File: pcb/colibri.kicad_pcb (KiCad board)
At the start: 2 copper layers, 160 x 95.2 mm, 97 parts

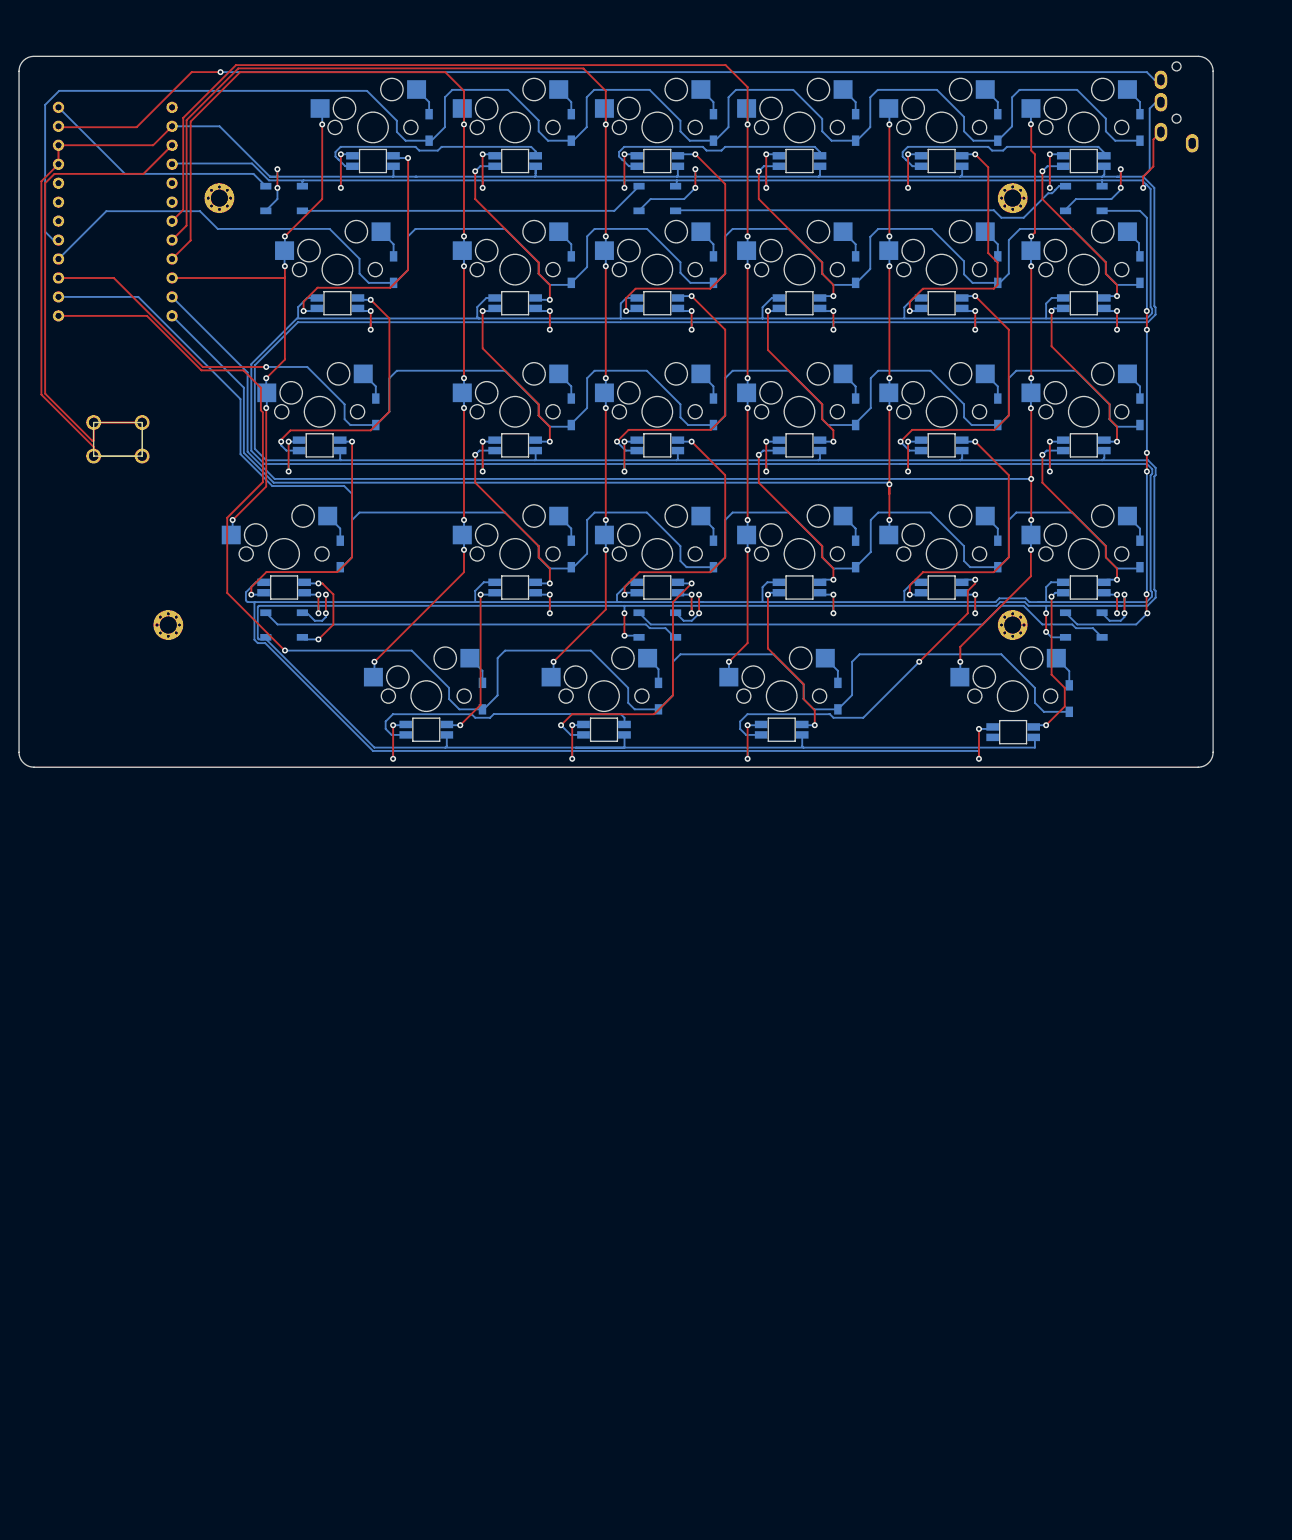
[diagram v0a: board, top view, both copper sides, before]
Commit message: starting to build the right side
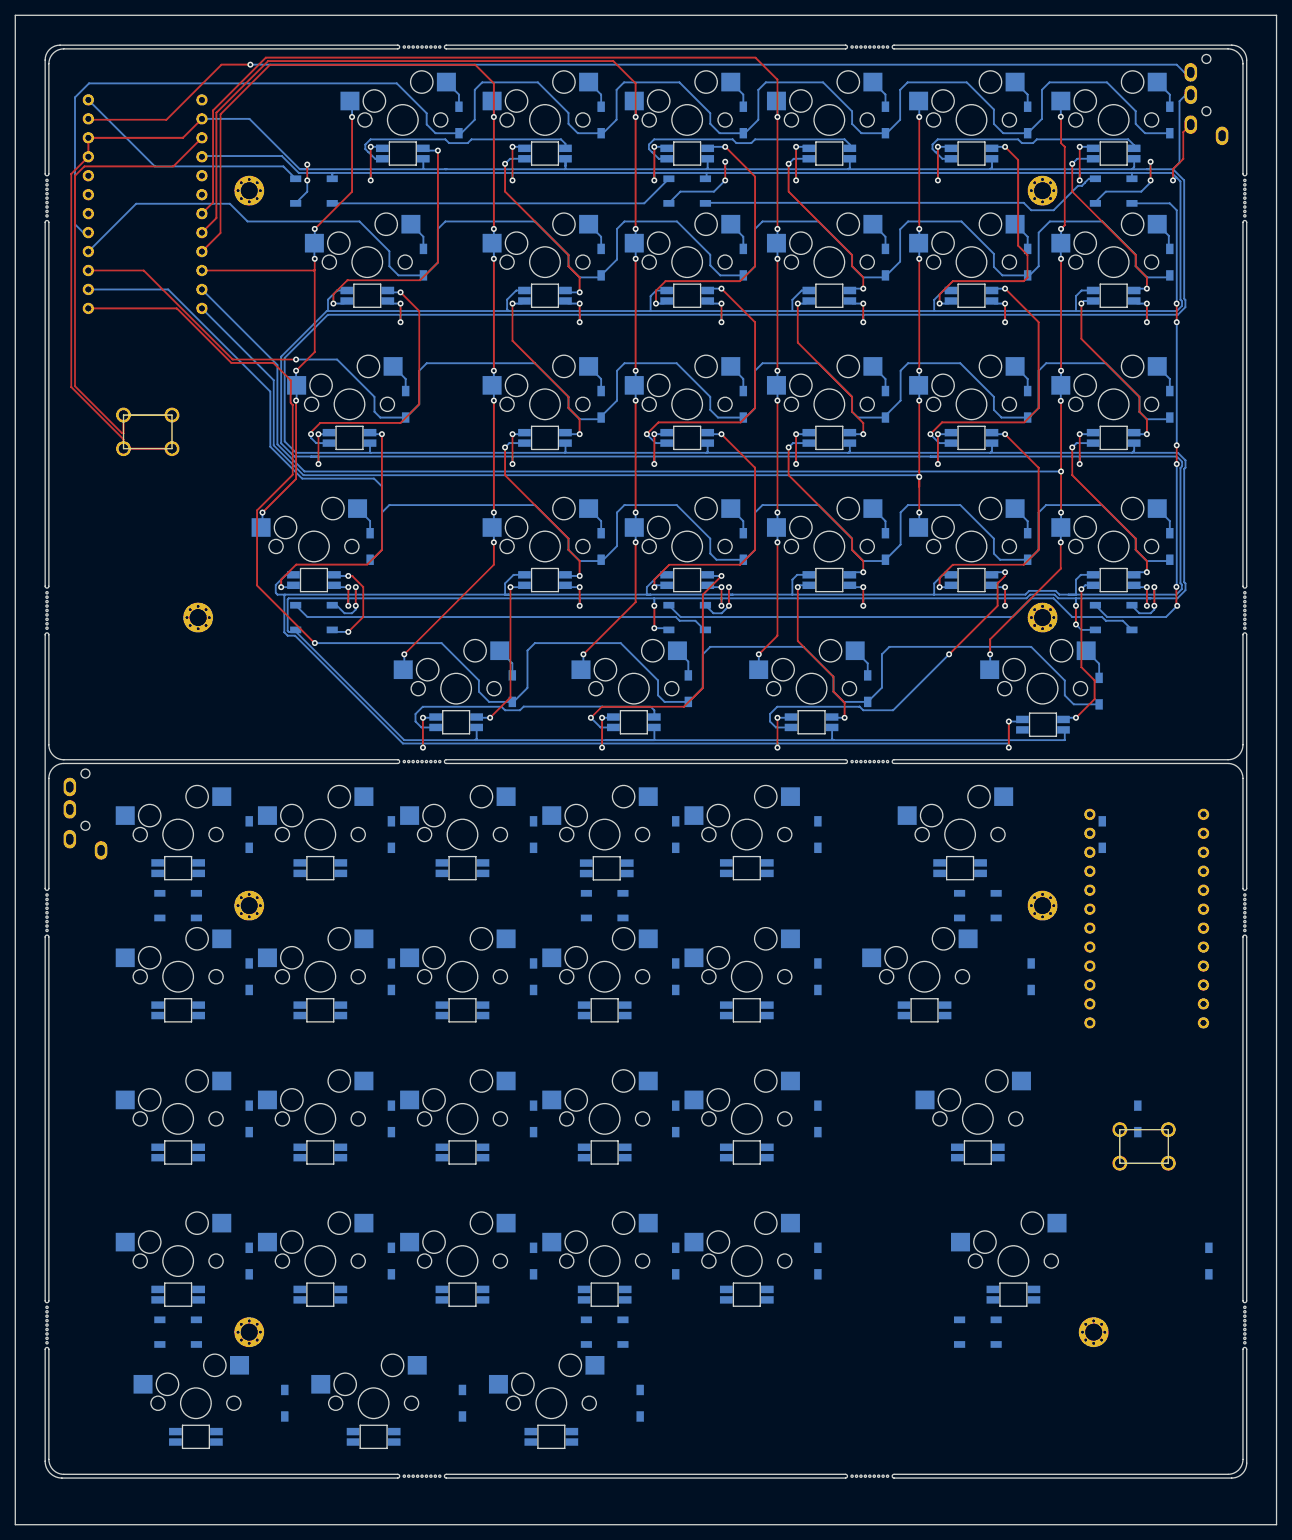
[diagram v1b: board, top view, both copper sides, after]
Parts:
- added REF**: Breakaway_Tabs, kbd:Breakaway_Tabs, F.Cu at (75.0, 134.5)
- added REF**: Breakaway_Tabs, kbd:Breakaway_Tabs, F.Cu at (75.0, 230.2)
- added REF**: Breakaway_Tabs, kbd:Breakaway_Tabs, F.Cu at (24.8, 114.2)
- added REF**: Breakaway_Tabs, kbd:Breakaway_Tabs, F.Cu at (75.0, 38.8)
- added REF**: Breakaway_Tabs, kbd:Breakaway_Tabs, F.Cu at (24.8, 210.0)
- added REF**: Breakaway_Tabs, kbd:Breakaway_Tabs, F.Cu at (24.8, 154.8)
- added REF**: Breakaway_Tabs, kbd:Breakaway_Tabs, F.Cu at (24.8, 59.0)
- added REF**: Breakaway_Tabs, kbd:Breakaway_Tabs, F.Cu at (135.0, 134.5)
- added REF**: Breakaway_Tabs, kbd:Breakaway_Tabs, F.Cu at (185.2, 114.2)
- added REF**: Breakaway_Tabs, kbd:Breakaway_Tabs, F.Cu at (185.2, 59.0)
- added REF**: Breakaway_Tabs, kbd:Breakaway_Tabs, F.Cu at (135.0, 38.8)
- added REF**: Breakaway_Tabs, kbd:Breakaway_Tabs, F.Cu at (185.2, 154.8)
- added REF**: Breakaway_Tabs, kbd:Breakaway_Tabs, F.Cu at (185.2, 210.0)
- added REF**: Breakaway_Tabs, kbd:Breakaway_Tabs, F.Cu at (135.0, 230.2)
- added Ref**: Val**, kbd:M2_HOLE_v3, F.Cu at (51.8, 210.9)
- added Ref**: Val**, kbd:M2_HOLE_v3, F.Cu at (51.8, 153.8)
- added Ref**: Val**, kbd:M2_HOLE_v3, F.Cu at (165.0, 210.9)
- added Ref**: Val**, kbd:M2_HOLE_v3, F.Cu at (158.2, 153.8)
- added pro-micro2: ProMicro, kbd:ProMicro_v4, B.Cu at (172.1, 156.1)
- added rd-1: 1N4148W, kbd:D3_SMD_v2, B.Cu at (166.1, 144.3)
- added rd-10: 1N4148W, kbd:D3_SMD_v2, B.Cu at (89.9, 163.3)
- added rd-11: 1N4148W, kbd:D3_SMD_v2, B.Cu at (70.9, 163.3)
- added rd-12: 1N4148W, kbd:D3_SMD_v2, B.Cu at (51.8, 163.3)
- added rd-13: 1N4148W, kbd:D3_SMD_v2, B.Cu at (170.9, 182.4)
- added rd-14: 1N4148W, kbd:D3_SMD_v2, B.Cu at (128.0, 182.4)
- added rd-15: 1N4148W, kbd:D3_SMD_v2, B.Cu at (109.0, 182.4)
- added rd-16: 1N4148W, kbd:D3_SMD_v2, B.Cu at (89.9, 182.4)
- added rd-17: 1N4148W, kbd:D3_SMD_v2, B.Cu at (70.9, 182.4)
- added rd-18: 1N4148W, kbd:D3_SMD_v2, B.Cu at (51.8, 182.4)
- added rd-19: 1N4148W, kbd:D3_SMD_v2, B.Cu at (180.4, 201.4)
- added rd-2: 1N4148W, kbd:D3_SMD_v2, B.Cu at (128.0, 144.3)
- added rd-20: 1N4148W, kbd:D3_SMD_v2, B.Cu at (128.0, 201.4)
- added rd-21: 1N4148W, kbd:D3_SMD_v2, B.Cu at (109.0, 201.4)
- added rd-22: 1N4148W, kbd:D3_SMD_v2, B.Cu at (89.9, 201.4)
- added rd-23: 1N4148W, kbd:D3_SMD_v2, B.Cu at (70.9, 201.4)
- added rd-24: 1N4148W, kbd:D3_SMD_v2, B.Cu at (51.8, 201.4)
- added rd-25: 1N4148W, kbd:D3_SMD_v2, B.Cu at (104.2, 220.5)
- added rd-26: 1N4148W, kbd:D3_SMD_v2, B.Cu at (80.4, 220.5)
- added rd-27: 1N4148W, kbd:D3_SMD_v2, B.Cu at (56.6, 220.5)
- added rd-3: 1N4148W, kbd:D3_SMD_v2, B.Cu at (109.0, 144.3)
- added rd-4: 1N4148W, kbd:D3_SMD_v2, B.Cu at (89.9, 144.3)
- added rd-5: 1N4148W, kbd:D3_SMD_v2, B.Cu at (70.9, 144.3)
- added rd-6: 1N4148W, kbd:D3_SMD_v2, B.Cu at (51.8, 144.3)
- added rd-7: 1N4148W, kbd:D3_SMD_v2, B.Cu at (156.6, 163.3)
- added rd-8: 1N4148W, kbd:D3_SMD_v2, B.Cu at (128.0, 163.3)
- added rd-9: 1N4148W, kbd:D3_SMD_v2, B.Cu at (109.0, 163.3)
- added rjack-1: MJ-4PP-9, kbd:MJ-4PP-9_1side, B.Cu at (29.9, 134.6)
- added rled-1: YS-SK6812MINI-E, kbd:YS-SK6812MINI-E, B.Cu at (147.1, 148.8)
- added rled-10: YS-SK6812MINI-E, kbd:YS-SK6812MINI-E, B.Cu at (80.4, 167.8)
- added rled-11: YS-SK6812MINI-E, kbd:YS-SK6812MINI-E, B.Cu at (61.4, 167.8)
- added rled-12: YS-SK6812MINI-E, kbd:YS-SK6812MINI-E, B.Cu at (42.3, 167.8)
- added rled-13: YS-SK6812MINI-E, kbd:YS-SK6812MINI-E, B.Cu at (149.5, 186.9)
- added rled-14: YS-SK6812MINI-E, kbd:YS-SK6812MINI-E, B.Cu at (118.5, 186.9)
- added rled-15: YS-SK6812MINI-E, kbd:YS-SK6812MINI-E, B.Cu at (99.5, 186.9)
- added rled-16: YS-SK6812MINI-E, kbd:YS-SK6812MINI-E, B.Cu at (80.4, 186.9)
- added rled-17: YS-SK6812MINI-E, kbd:YS-SK6812MINI-E, B.Cu at (61.4, 186.9)
- added rled-18: YS-SK6812MINI-E, kbd:YS-SK6812MINI-E, B.Cu at (42.3, 186.9)
- added rled-19: YS-SK6812MINI-E, kbd:YS-SK6812MINI-E, B.Cu at (154.2, 205.9)
- added rled-2: YS-SK6812MINI-E, kbd:YS-SK6812MINI-E, B.Cu at (118.5, 148.8)
- added rled-20: YS-SK6812MINI-E, kbd:YS-SK6812MINI-E, B.Cu at (118.5, 205.9)
- added rled-21: YS-SK6812MINI-E, kbd:YS-SK6812MINI-E, B.Cu at (99.5, 205.9)
- added rled-22: YS-SK6812MINI-E, kbd:YS-SK6812MINI-E, B.Cu at (80.4, 205.9)
- added rled-23: YS-SK6812MINI-E, kbd:YS-SK6812MINI-E, B.Cu at (61.4, 205.9)
- added rled-24: YS-SK6812MINI-E, kbd:YS-SK6812MINI-E, B.Cu at (42.3, 205.9)
- added rled-25: YS-SK6812MINI-E, kbd:YS-SK6812MINI-E, B.Cu at (92.3, 225.0)
- added rled-26: YS-SK6812MINI-E, kbd:YS-SK6812MINI-E, B.Cu at (68.5, 225.0)
- added rled-27: YS-SK6812MINI-E, kbd:YS-SK6812MINI-E, B.Cu at (44.7, 225.0)
- added rled-3: YS-SK6812MINI-E, kbd:YS-SK6812MINI-E, B.Cu at (99.8, 148.8)
- added rled-4: YS-SK6812MINI-E, kbd:YS-SK6812MINI-E, B.Cu at (80.4, 148.8)
- added rled-5: YS-SK6812MINI-E, kbd:YS-SK6812MINI-E, B.Cu at (61.4, 148.8)
- added rled-6: YS-SK6812MINI-E, kbd:YS-SK6812MINI-E, B.Cu at (42.3, 148.8)
- added rled-7: YS-SK6812MINI-E, kbd:YS-SK6812MINI-E, B.Cu at (142.3, 167.8)
- added rled-8: YS-SK6812MINI-E, kbd:YS-SK6812MINI-E, B.Cu at (118.5, 167.8)
- added rled-9: YS-SK6812MINI-E, kbd:YS-SK6812MINI-E, B.Cu at (99.5, 167.8)
- added rreset-1: SW_PUSH, kbd:ResetSW_4P, B.Cu at (171.8, 186.1)
- added rsw-1: SW_PUSH, kbd:CherryMX_Hotswap_2u, F.Cu at (147.1, 144.3)
- added rsw-10: SW_PUSH, kbd:CherryMX_Hotswap, F.Cu at (80.4, 163.3)
- added rsw-11: SW_PUSH, kbd:CherryMX_Hotswap, F.Cu at (61.4, 163.3)
- added rsw-12: SW_PUSH, kbd:CherryMX_Hotswap, F.Cu at (42.3, 163.3)
- added rsw-13: SW_PUSH, kbd:CherryMX_Hotswap_2.25u, F.Cu at (149.5, 182.4)
- added rsw-14: SW_PUSH, kbd:CherryMX_Hotswap, F.Cu at (118.5, 182.4)
- added rsw-15: SW_PUSH, kbd:CherryMX_Hotswap, F.Cu at (99.5, 182.4)
- added rsw-16: SW_PUSH, kbd:CherryMX_Hotswap, F.Cu at (80.4, 182.4)
- added rsw-17: SW_PUSH, kbd:CherryMX_Hotswap, F.Cu at (61.4, 182.4)
- added rsw-18: SW_PUSH, kbd:CherryMX_Hotswap, F.Cu at (42.3, 182.4)
- added rsw-19: SW_PUSH, kbd:CherryMX_Hotswap_2.75u, F.Cu at (154.2, 201.4)
- added rsw-2: SW_PUSH, kbd:CherryMX_Hotswap, F.Cu at (118.5, 144.3)
- added rsw-20: SW_PUSH, kbd:CherryMX_Hotswap, F.Cu at (118.5, 201.4)
- added rsw-21: SW_PUSH, kbd:CherryMX_Hotswap, F.Cu at (99.5, 201.4)
- added rsw-22: SW_PUSH, kbd:CherryMX_Hotswap, F.Cu at (80.4, 201.4)
- added rsw-23: SW_PUSH, kbd:CherryMX_Hotswap, F.Cu at (61.4, 201.4)
- added rsw-24: SW_PUSH, kbd:CherryMX_Hotswap, F.Cu at (42.3, 201.4)
- added rsw-25: SW_PUSH, kbd:CherryMX_Hotswap_1.25u, F.Cu at (92.3, 220.5)
- added rsw-26: SW_PUSH, kbd:CherryMX_Hotswap_1.25u, F.Cu at (68.5, 220.5)
- added rsw-27: SW_PUSH, kbd:CherryMX_Hotswap_1.25u, F.Cu at (44.7, 220.5)
- added rsw-3: SW_PUSH, kbd:CherryMX_Hotswap, F.Cu at (99.5, 144.3)
- added rsw-4: SW_PUSH, kbd:CherryMX_Hotswap, F.Cu at (80.4, 144.3)
- added rsw-5: SW_PUSH, kbd:CherryMX_Hotswap, F.Cu at (61.4, 144.3)
- added rsw-6: SW_PUSH, kbd:CherryMX_Hotswap, F.Cu at (42.3, 144.3)
- added rsw-7: SW_PUSH, kbd:CherryMX_Hotswap_1.5u, F.Cu at (142.3, 163.3)
- added rsw-8: SW_PUSH, kbd:CherryMX_Hotswap, F.Cu at (118.5, 163.3)
- added rsw-9: SW_PUSH, kbd:CherryMX_Hotswap, F.Cu at (99.5, 163.3)
- added ru-1: WS2812B, LED_SMD:LED_WS2812B_PLCC4_5.0x5.0mm_P3.2mm, B.Cu at (149.5, 153.8)
- added ru-2: WS2812B, LED_SMD:LED_WS2812B_PLCC4_5.0x5.0mm_P3.2mm, B.Cu at (99.5, 153.8)
- added ru-3: WS2812B, LED_SMD:LED_WS2812B_PLCC4_5.0x5.0mm_P3.2mm, B.Cu at (42.3, 153.8)
- added ru-4: WS2812B, LED_SMD:LED_WS2812B_PLCC4_5.0x5.0mm_P3.2mm, B.Cu at (149.5, 210.9)
- added ru-5: WS2812B, LED_SMD:LED_WS2812B_PLCC4_5.0x5.0mm_P3.2mm, B.Cu at (99.5, 210.9)
- added ru-6: WS2812B, LED_SMD:LED_WS2812B_PLCC4_5.0x5.0mm_P3.2mm, B.Cu at (42.3, 210.9)
- moved Ref** 4.12 mm to (45.0, 115.2)
- moved Ref** 4.12 mm to (51.9, 58.0)
- moved Ref** 4.12 mm to (158.2, 115.2)
- moved Ref** 4.12 mm to (158.2, 58.0)
- moved ld-1 4.12 mm to (80.0, 48.5)
- moved ld-10 4.12 mm to (137.1, 67.6)
- moved ld-11 4.12 mm to (156.2, 67.6)
- moved ld-12 4.12 mm to (175.2, 67.6)
- moved ld-13 4.12 mm to (72.8, 86.6)
- moved ld-14 4.12 mm to (99.0, 86.6)
- moved ld-15 4.12 mm to (118.0, 86.6)
- moved ld-16 4.12 mm to (137.1, 86.6)
- moved ld-17 4.12 mm to (156.2, 86.6)
- moved ld-18 4.12 mm to (175.2, 86.6)
- moved ld-19 4.12 mm to (68.0, 105.7)
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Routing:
- net lVCC: track 853.0 -> 849.0 mm
- net lGND: track 877.6 -> 876.9 mm
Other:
- board size 160 x 95.2 mm -> 169 x 202.2 mm
